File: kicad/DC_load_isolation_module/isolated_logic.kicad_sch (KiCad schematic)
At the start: 23 parts, among them Q18 MMBT5401, Q2 MMBT5401, Q3 MMBT5401, Q4 MMBT5551L, Q7 MMBT5551L, U1 LTV-817S, U3 LTV-817S, U4 LTV-817S

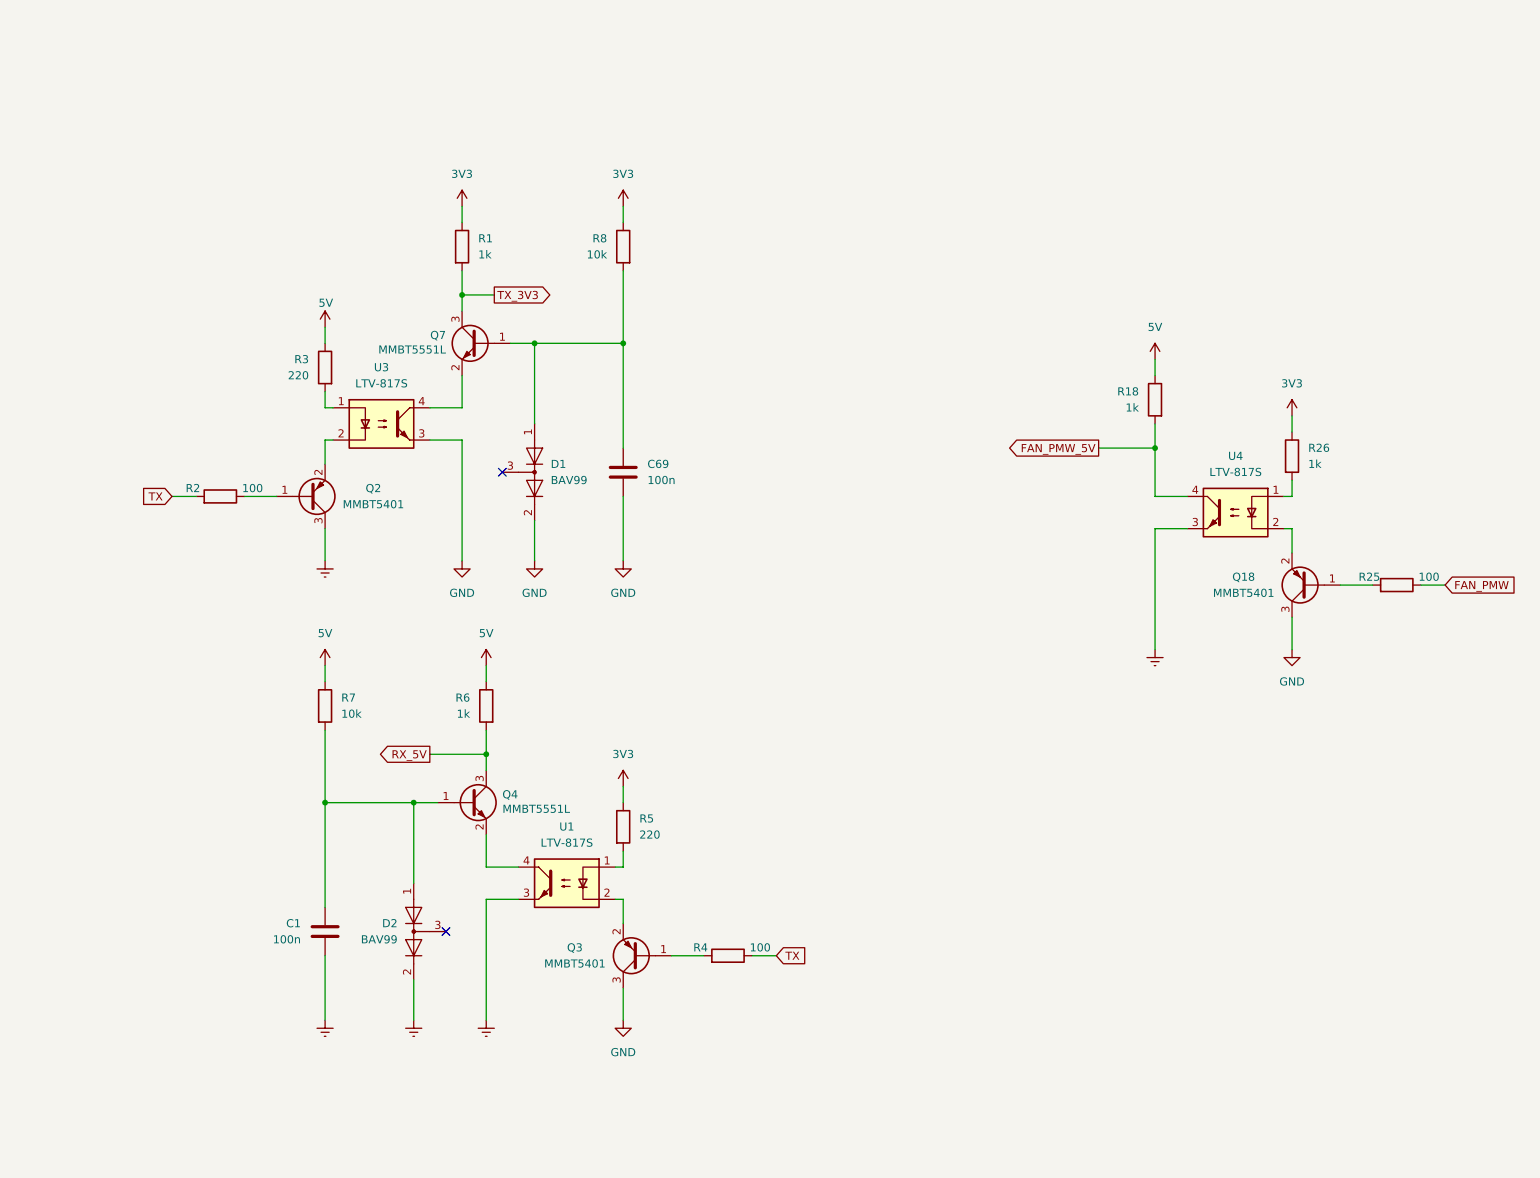
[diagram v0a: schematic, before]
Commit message: Schematic done.
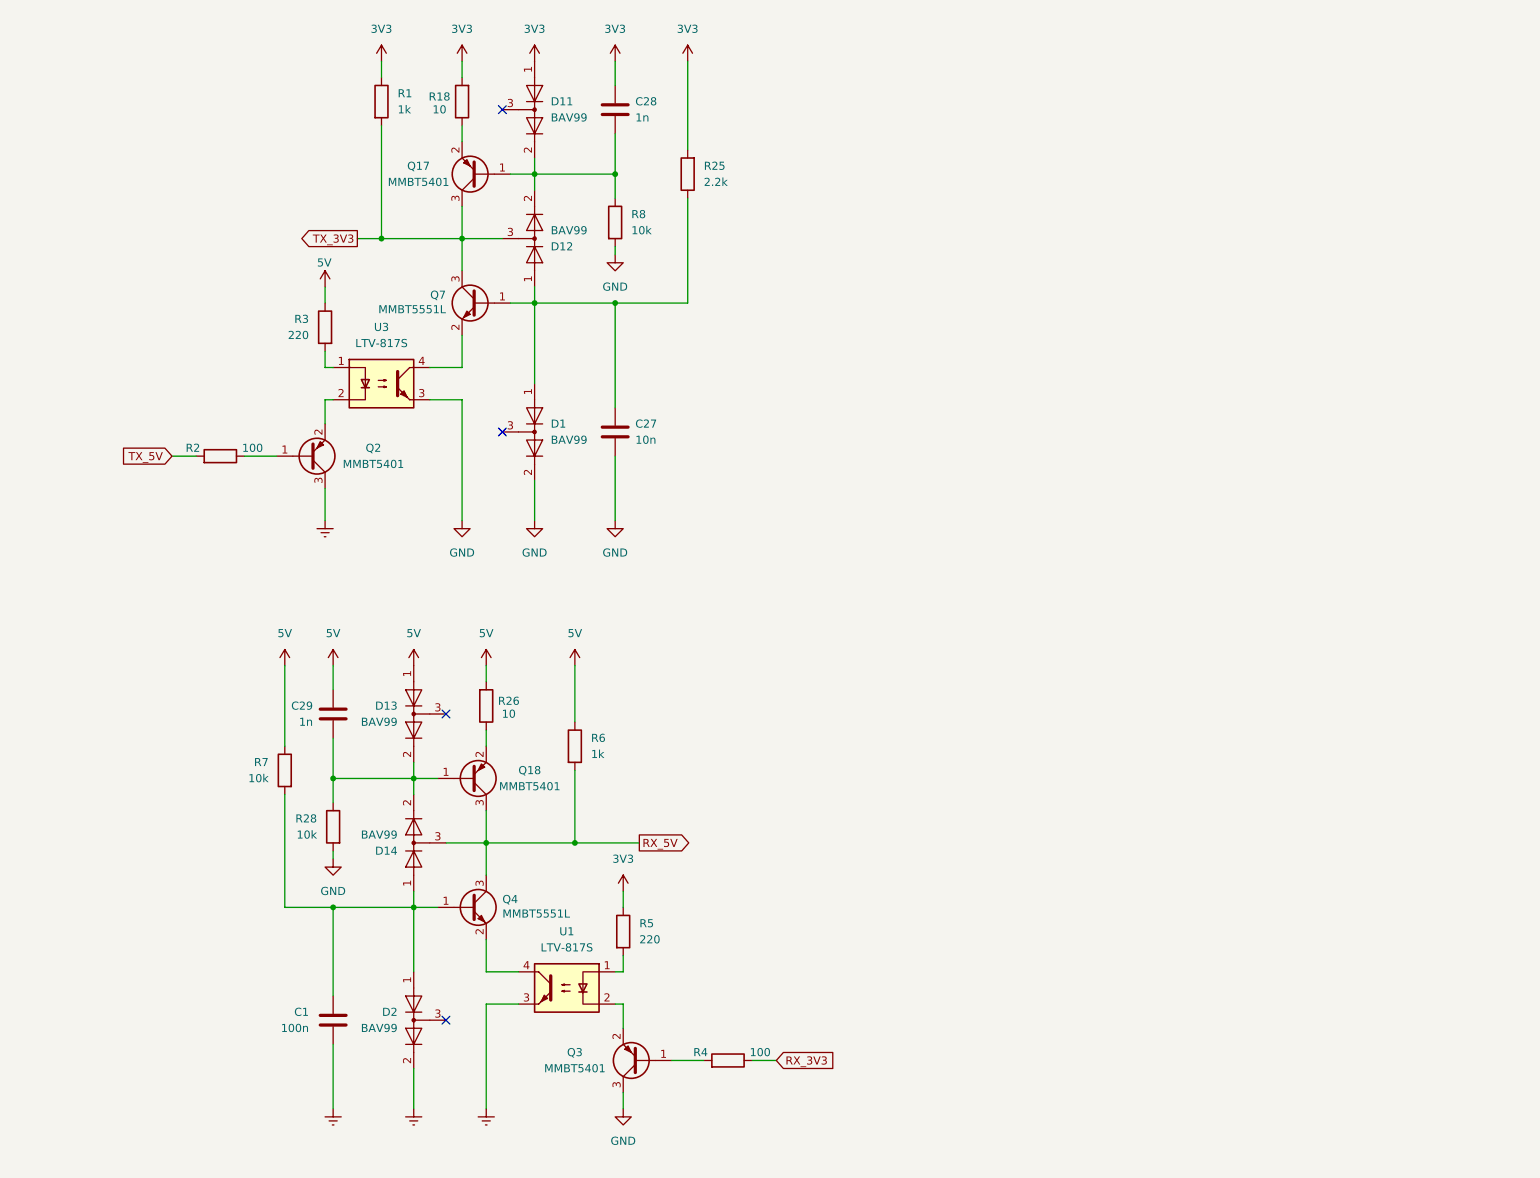
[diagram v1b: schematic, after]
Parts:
- removed C69: 100n, Capacitor_SMD:C_0603_1608Metric_Pad1.08x0.95mm_HandSolder, symbol Device:C
- removed U4: LTV-817S, Package_DIP:SMDIP-4_W9.53mm, symbol Isolator:LTV-817S
- added C27: 10n, Capacitor_SMD:C_0603_1608Metric_Pad1.08x0.95mm_HandSolder, symbol Device:C
- added C28, C29: 1n, Capacitor_SMD:C_0603_1608Metric_Pad1.08x0.95mm_HandSolder, symbol Device:C
- added D11, D12, D13, D14: BAV99, Package_TO_SOT_SMD:SOT-23, symbol Diode:BAV99
- added Q17: MMBT5401, Package_TO_SOT_SMD:SOT-23, symbol Transistor_BJT:MMBT3906
- added R28: 10k, Resistor_SMD:R_0603_1608Metric_Pad0.98x0.95mm_HandSolder, symbol Device:R
- R18, R26: value 1k -> 10; LCSC C22962 -> C22859
- R25: value 100 -> 2.2k; LCSC C22775 -> C4190
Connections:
- net FAN_PMW is gone; now on an unnamed net: R25.1
- net FAN_PMW_5V is gone; now on net 3V3: R18.2
- net 3V3: now also R25.2, C28.2, D11.1 (K); no longer R26.1, R8.1
- net 5V: now also R26.2, C29.2, D13.1 (K); no longer R18.1
- net GND: now also R8.2, C27.1, R28.2; no longer Q18.3 (C)
- net RX_5V: now also Q18.3 (C), D14.3 (K)
- net TX_3V3: now also D12.3 (K), Q17.3 (C)
- net at C1.2, D2.1 (K), Q4.1 (B)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: now also D14.1 (K)
- net at Q18.1 (B): now also C29.1, D13.2 (A), D14.2 (A), R28.1; no longer R25.2
- net at Q18.2 (E): now also R26.1
- net at D1.1 (K), Q7.1 (B): now also C27.2, D12.1 (K); no longer R8.2
- net TX renamed RX_3V3
- net RX_3V3: no longer R2.2
- new net: C28.1, D11.2 (A), D12.2 (A), Q17.1 (B), R8.1
- new net: Q17.2 (E), R18.1
- new net TX_5V: R2.2
- no-connect marks 2 -> 4
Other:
- moved on the sheet: C1, D1, D2, Q2, Q3, Q4, Q7, R1, R2, R3, R4, R5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

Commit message: M
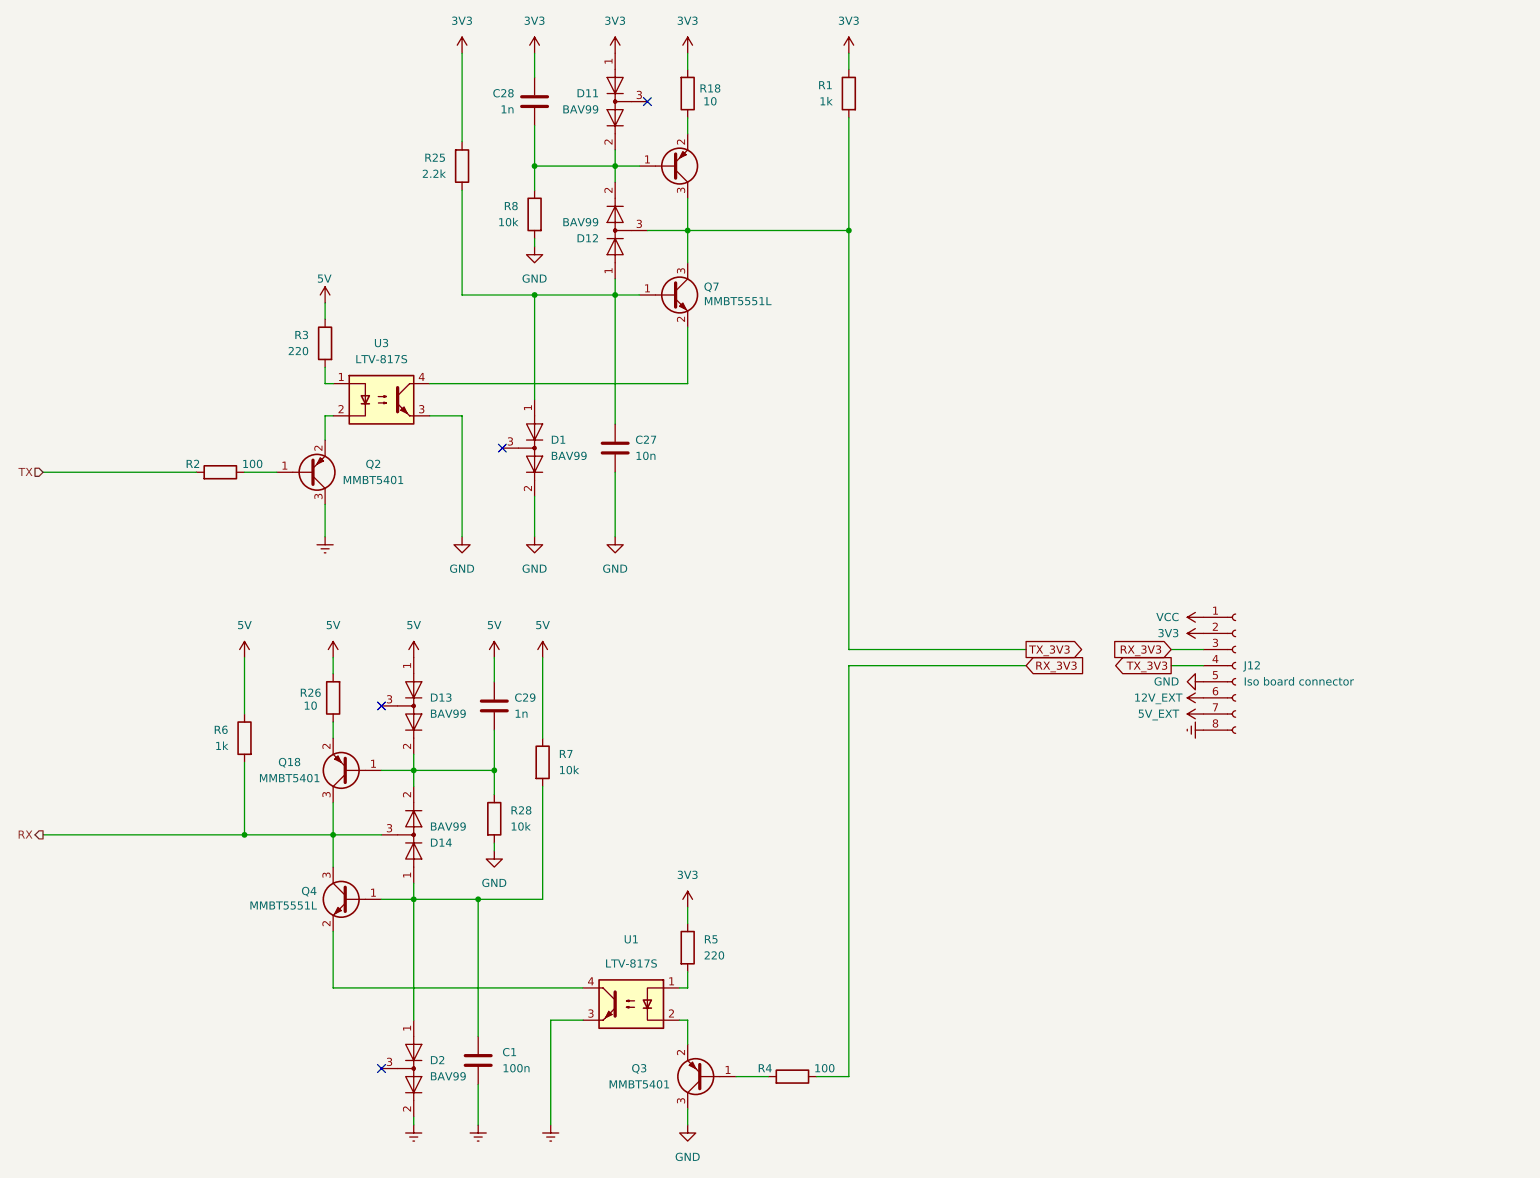
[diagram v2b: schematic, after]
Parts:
- added J12: Iso board connector, Connector_PinSocket_2.54mm:PinSocket_1x08_P2.54mm_Vertical, symbol Connector:Conn_01x08_Socket
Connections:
- net 3V3: now also J12.2 (Pin_2)
- net Earth: now also J12.8 (Pin_8)
- net GND: now also J12.5 (Pin_5)
- net RX_3V3: now also J12.3 (Pin_3)
- net TX_3V3: now also J12.4 (Pin_4)
- net RX_5V renamed RX
- net TX_5V renamed TX
- new net 12V_EXT: J12.6 (Pin_6)
- new net 5V_EXT: J12.7 (Pin_7)
- new net VCC: J12.1 (Pin_1)
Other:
- moved on the sheet: C1, C27, C28, C29, D1, D11, D12, D13, D14, D2, Q18, Q2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

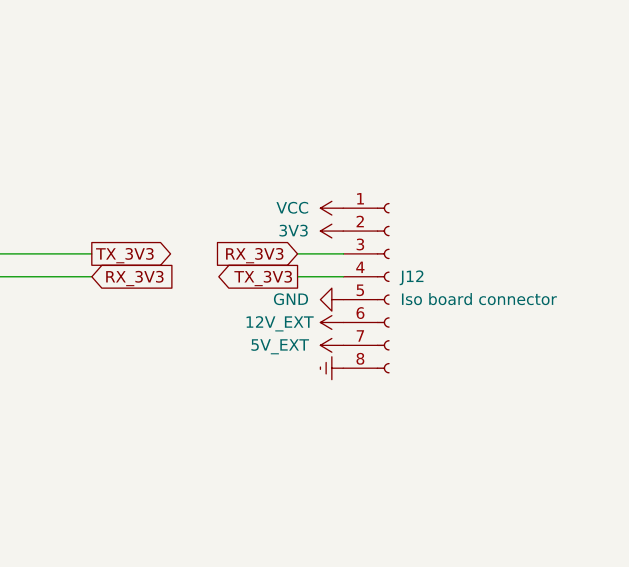
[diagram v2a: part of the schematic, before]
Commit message: SRF layout
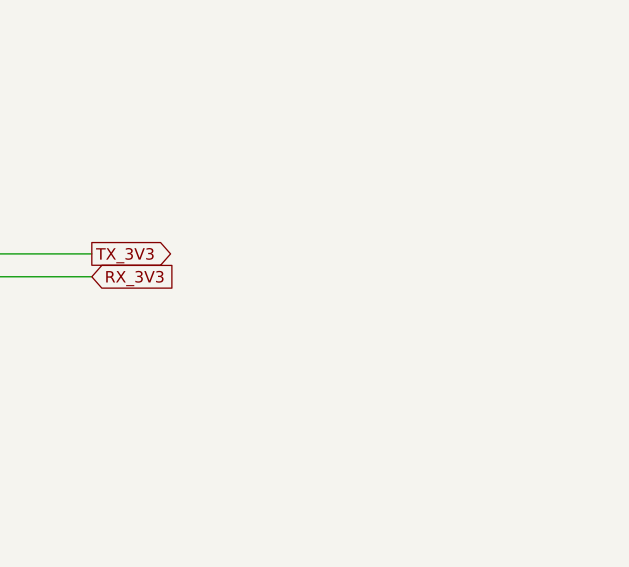
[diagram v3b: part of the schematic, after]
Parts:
- removed J12: Iso board connector, Connector_PinSocket_2.54mm:PinSocket_1x08_P2.54mm_Vertical, symbol Connector:Conn_01x08_Socket
